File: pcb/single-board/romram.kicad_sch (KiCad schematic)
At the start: 26 parts, among them U10 74HC273, U11 74HC273, U12 74HC245, U13 74HC245, U14 74HC10, U15 SST39SF040, U16 AS6C4008, U17 CY62256, U5 74HC688, U6 74HC688, U7 74HC04, U8 74HC10, U9 74HC00

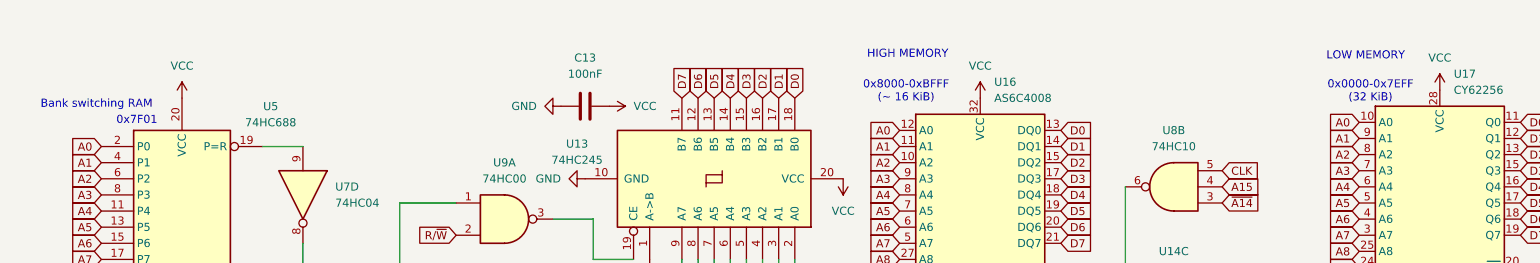
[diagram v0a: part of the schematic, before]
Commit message: Further revising
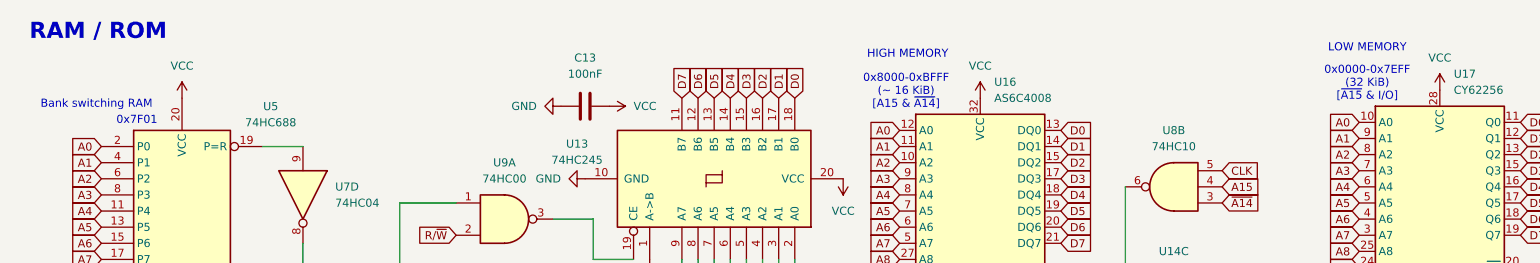
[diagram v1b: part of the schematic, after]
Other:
- note added: "0x0000-0x7EFF (32 KiB) [~{A15} & I/O]"
- note added: "0x8000-0xBFFF (~ 16 KiB) [A15 & ~{A14}]"
- note added: "RAM / ROM"
- note removed: "0x0000-0x7EFF (32 KiB)"
- note removed: "0x8000-0xBFFF (~ 16 KiB)"
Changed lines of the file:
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@@
 		)
 	)
-	(text "0x8000-0xBFFF\n(~ 16 KiB)"
+	(text "0x8000-0xBFFF\n(~ 16 KiB)\n[A15 & ~{A14}]"
 		(exclude_from_sim no)
 		(at 152.146 25.654 0)
@@
 	(text "LOW MEMORY"
 		(exclude_from_sim no)
-		(at 224.536 20.066 0)
+		(at 224.79 18.796 0)
 		(effects
 			(font
@@
 		)
 	)
+	(text "RAM / ROM"
+		(exclude_from_sim no)
+		(at 24.892 16.256 0)
+		(effects
+			(font
+				(size 2.54 2.54)
+				(thickness 0.508)
+				(bold yes)
+			)
+		)
+	)
 	(text "Latch LOW-to-HIGH\nHappens when CLK goes low"
 		(exclude_from_sim no)
@@
 		)
 	)
-	(text "0x0000-0x7EFF\n(32 KiB)"
+	(text "0x0000-0x7EFF\n(32 KiB)\n[~{A15} & I/O]"
 		(exclude_from_sim no)
-		(at 225.298 25.654 0)
+		(at 224.79 24.384 0)
 		(effects
 			(font
